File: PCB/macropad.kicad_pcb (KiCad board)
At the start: 2 copper layers, 81.1 x 93.4 mm, 38 parts, among them SW1 SW_Push, SW10 SW_Push, SW11 SW_Push, SW12 SW_Push, SW13 SW_Push, SW14 SW_Push, SW15 SW_Push, SW16 SW_Push, SW2 SW_Push, SW3 SW_Push, SW4 SW_Push, SW5 SW_Push, SW6 SW_Push, SW7 SW_Push, SW8 SW_Push, SW9 SW_Push, U2 MOUDLE-SEEEDUINO-XIAO

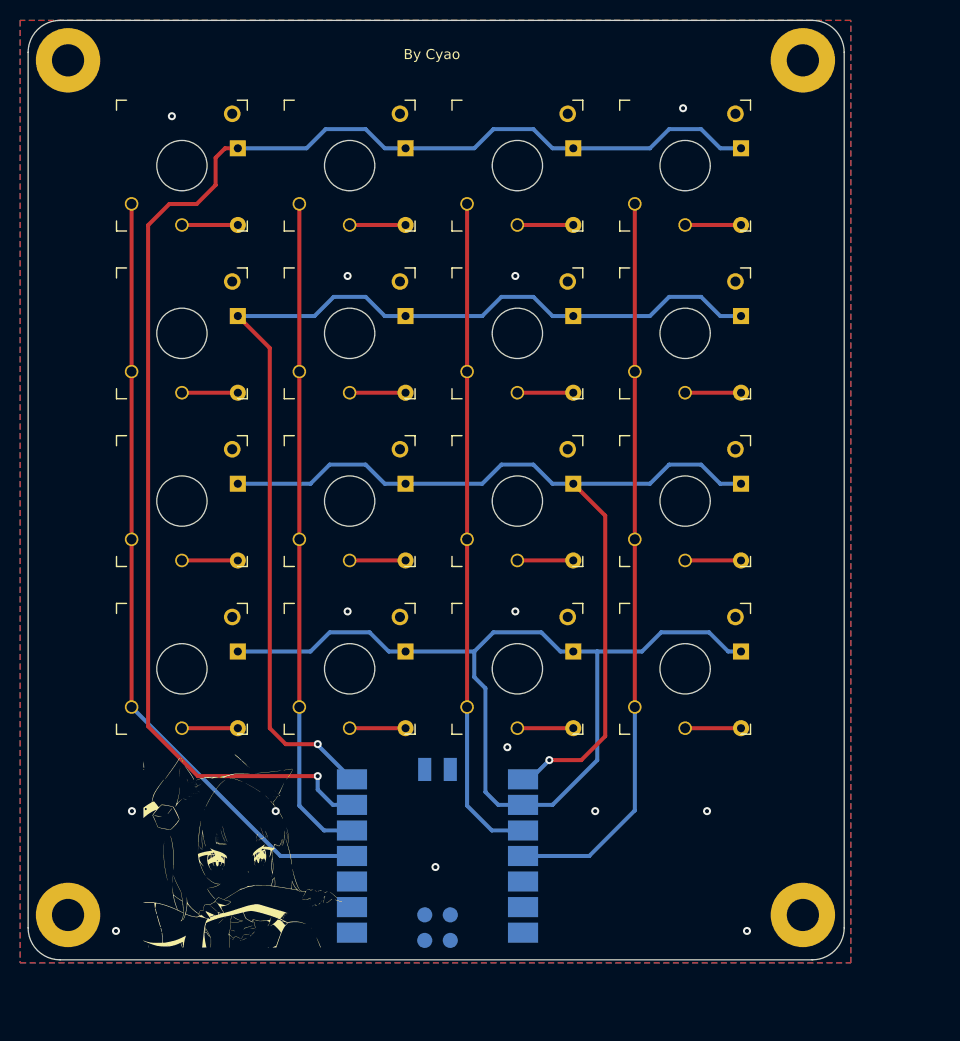
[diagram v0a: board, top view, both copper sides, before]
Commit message: LCD!
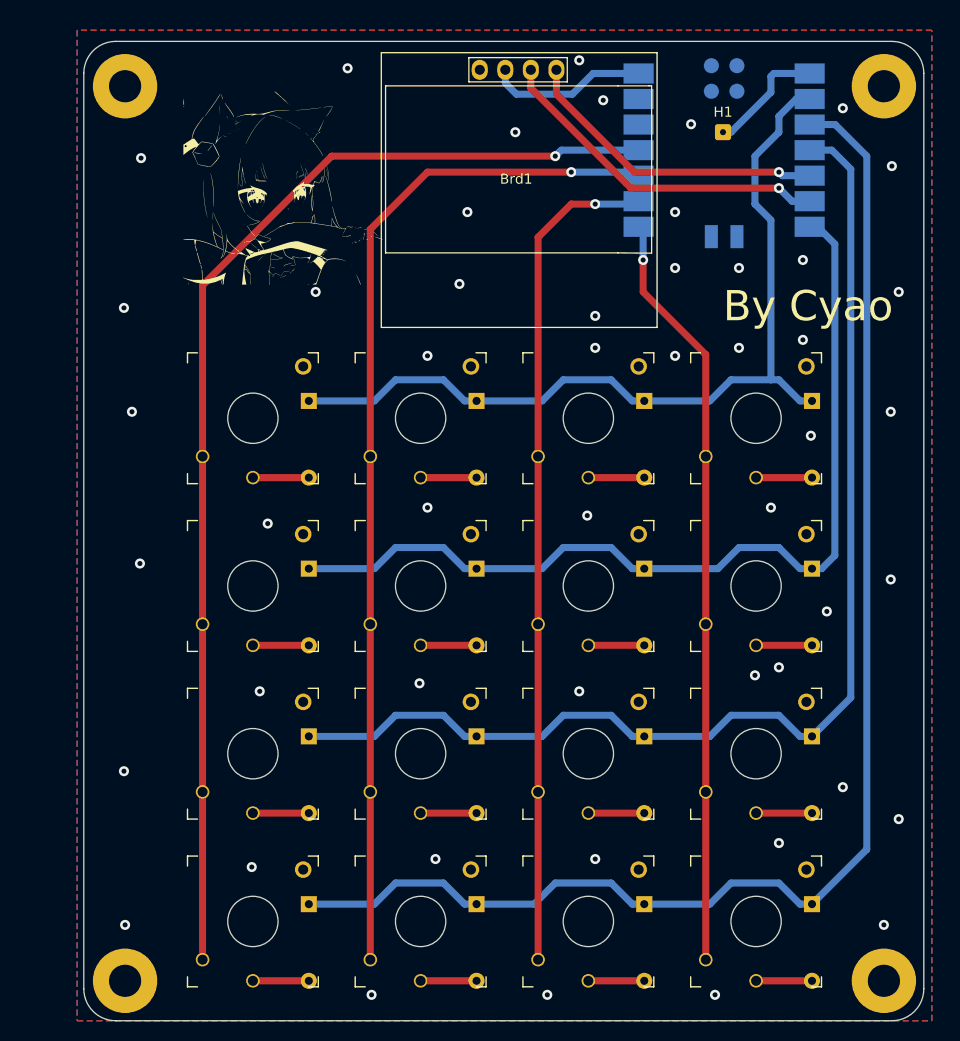
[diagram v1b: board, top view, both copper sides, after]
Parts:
- added Brd1: SSD1306, screen:128x64OLED, F.Cu at (163.6, 63.1)
- added H1: MountingHole_Pad, Connector_Wire:SolderWire-0.1sqmm_1x01_D0.4mm_OD1mm, F.Cu at (184.2, 58.7)
- moved ? 122.2 mm to (200.1, 143.1), turned to 180 degrees
- moved ? 115.6 mm to (200.1, 54.2), turned to 0 degrees
- moved REF** 113.6 mm to (124.7, 143.1), turned to 180 degrees
- moved ? 106.4 mm to (124.7, 54.2), turned to 180 degrees
- moved U2 75.7 mm to (184.3, 60.5), turned to 180 degrees
- moved Gura! 66.0 mm to (140.5, 64.3)
- moved D1 26.1 mm to (143.0, 85.4)
- moved D10 26.1 mm to (193.0, 85.4)
- moved D11 26.1 mm to (193.0, 102.1)
- moved D12 26.1 mm to (193.0, 118.8)
- moved D2 26.1 mm to (159.7, 85.4)
- moved D4 26.1 mm to (143.0, 102.1)
- moved D5 26.1 mm to (159.7, 102.1)
- moved D7 26.1 mm to (143.0, 118.8)
- moved D8 26.1 mm to (159.7, 118.8)
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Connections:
- U2 pad 1: unconnected-(U2-PA02_A0_D0-Pad1) -> Net-(U2-PA02_A0_D0)
- U2 pad 10: COL2 -> COL1
- U2 pad 11: COL3 -> COL0
- U2 pad 2: unconnected-(U2-PA4_A1_D1-Pad2) -> ROW0
- U2 pad 3: unconnected-(U2-PA10_A2_D2-Pad3) -> ROW3
- U2 pad 4: COL0 -> ROW2
- U2 pad 5: COL1 -> Net-(Brd1-SDA)
- U2 pad 6: ROW0 -> Net-(Brd1-SCL)
- U2 pad 8: ROW2 -> COL3
- U2 pad 9: ROW3 -> COL2
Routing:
- net ROW0: track 142.5 -> 86.8 mm, vias 1 -> 0
- net ROW3: track 93.4 -> 138.8 mm
- net COL0: track 78.0 -> 115.9 mm, vias 0 -> 1
- net COL1: track 66.1 -> 101.7 mm, vias 0 -> 1
- net Net-(Brd1-SCL): track 0.00 -> 34.6 mm, vias 0 -> 1
- net Net-(Brd1-SDA): track 0.00 -> 31.2 mm, vias 0 -> 1
- net ROW2: track 91.1 -> 118.1 mm, vias 1 -> 0
- net COL2: track 66.4 -> 83.3 mm, vias 0 -> 1
- net +5V: track 0.00 -> 15.9 mm
- net ROW1: track 107.3 -> 92.2 mm, vias 1 -> 0
- net Net-(U2-PA02_A0_D0): track 0.00 -> 12.0 mm
- net COL3: track 73.3 -> 75.6 mm, vias 0 -> 1
- net GND: vias 14 -> 50
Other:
- board size 81.1 x 93.4 mm -> 83.5 x 97.3 mm
- board text removed: "UwU"
